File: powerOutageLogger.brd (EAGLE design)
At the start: 99.1 x 74.9 mm, 32 parts, among them J1 2.1MMJACKTHM, U1 ATmega328P, U2 78L05, Y1 16MHz

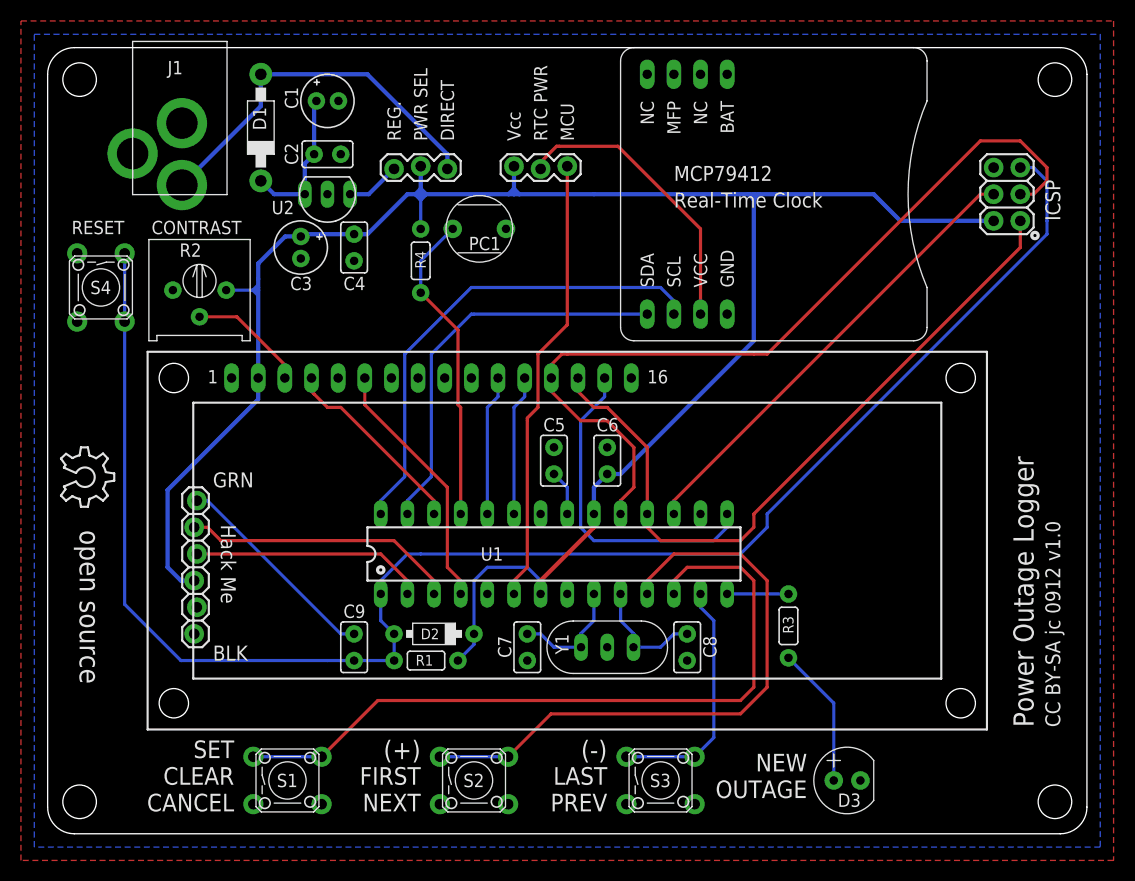
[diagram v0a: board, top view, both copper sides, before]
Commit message: v1.1
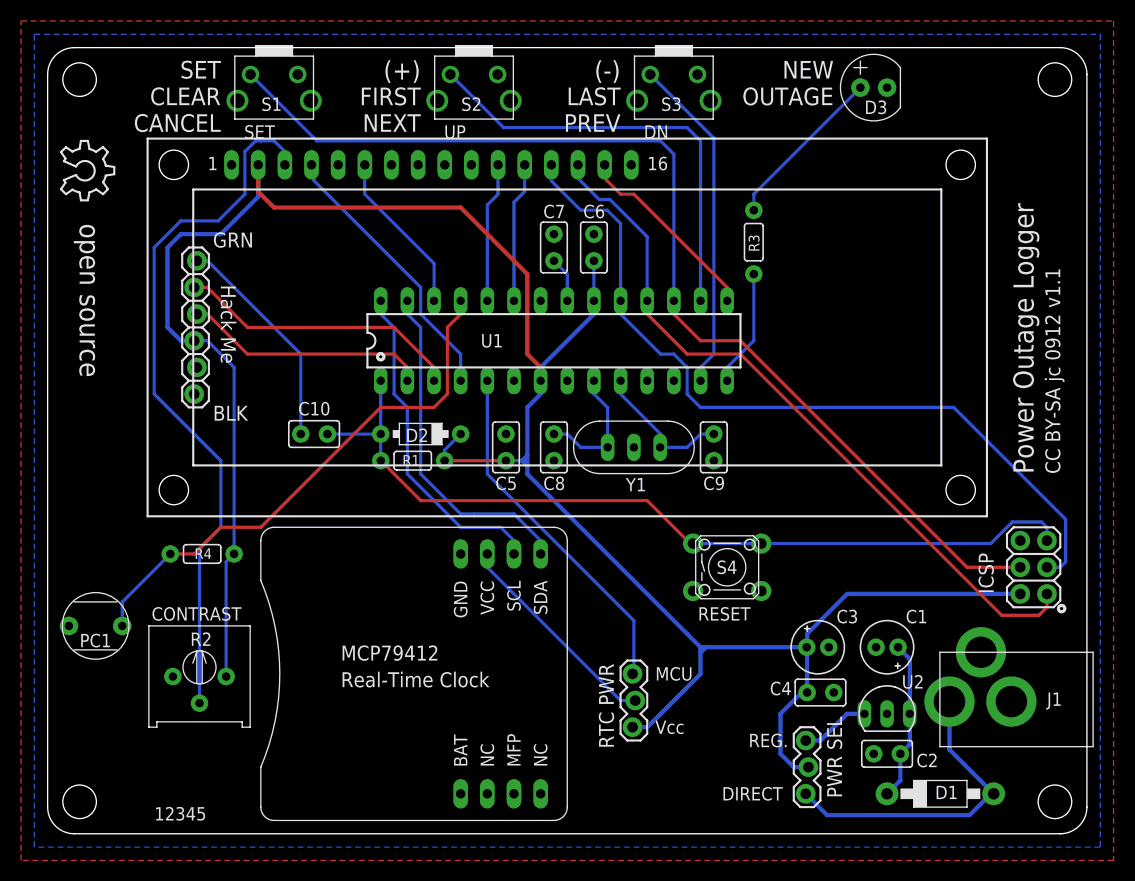
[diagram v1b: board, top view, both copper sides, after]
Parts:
- added C10: 100nF, _jc:C025-025X050
- added U$2: (no value), ohw-logo:OSHW_8X200_NOTEXT
- C7: value 27pF -> 100nF
- C9: value 100nF -> 27pF
- S1, S2: device _jc:B3F-10XXOCT -> _jc:B3F-312X
- S3: value DOWN -> DN; device _jc:B3F-10XXOCT -> _jc:B3F-312X
- moved J1 101.1 mm to (95.2, 12.7), turned to 270 degrees
- moved D1 90.7 mm to (85.1, 3.81), turned to 0 degrees
- moved C2 78.2 mm to (80.0, 7.62), turned to 180 degrees
- moved C1 74.5 mm to (80.0, 17.8), turned to 180 degrees
- moved U2 72.8 mm to (80.0, 11.4), turned to 0 degrees
- moved JP1 68.8 mm to (72.4, 3.81), turned to 90 degrees
- moved D3 66.1 mm to (78.7, 71.1)
- moved S1 66.1 mm to (21.6, 71.1)
- moved S3 66.1 mm to (59.7, 71.1)
- moved S2 66.0 mm to (40.6, 71.1)
- moved S4 65.4 mm to (64.8, 25.4), turned to 0 degrees
- moved C3 62.3 mm to (73.4, 17.8), turned to 0 degrees
- moved C4 61.4 mm to (73.7, 13.5), turned to 0 degrees
- moved PCB1 56.4 mm to (35.6, 15.2), turned to 90 degrees
- moved JP2 54.6 mm to (55.9, 10.2), turned to 90 degrees
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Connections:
- removed net PD4: JP2.3, U1.6
- removed net PD5: S2.1, S2.2, U1.11
- removed net PD6: S1.1, S1.2, U1.12
- net /RESET: now also C10.1; no longer C9.1
- net GND: now also C9.2, S1.1, S2.1, S3.1; no longer S1.3, S1.4, S2.3, S2.4, S3.3, S3.4
- net MOSI: now also S1.2
- net N$9: now also C7.1; no longer C5.1
- net PC3: now also PCB2.6; no longer PCB2.4
- net PD2: now also PCB2.4; no longer PCB2.6
- net PD3: now also JP2.3
- net PD7: no longer S3.1
- net RST: now also C10.2; no longer C9.2
- net SS: now also S2.2
- net VCC: now also C5.1
- net XTAL1: now also C9.1; no longer C8.1
- net XTAL2: now also C8.1; no longer C7.1
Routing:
- net /RESET: track 155.6 -> 81.8 mm
- net PD6: track 70.5 -> 0.00 mm
- net PD5: track 58.9 -> 0.00 mm
- net MOSI: track 43.8 -> 101.8 mm
- net N$3: track 11.3 -> 67.8 mm
- net PD4: track 42.9 -> 0.00 mm
- net SS: track 0.00 -> 41.7 mm
- net PD3: track 0.00 -> 33.9 mm
- net VCC: track 192.7 -> 219.8 mm
- net PC2: track 30.0 -> 50.9 mm
- net SCL: track 46.3 -> 31.6 mm
- net PB1: track 31.5 -> 18.5 mm
- net PD7: track 23.3 -> 32.2 mm
- net N$5: track 27.9 -> 20.6 mm
- net SDA: track 38.3 -> 32.4 mm
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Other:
- board text added: "12345"
- board text added: "CC BY-SA jc 0912 v1.1"
- board text added: "http://github.com/JChristensen"
- board text removed: "CC BY-SA jc 0912 v1.0"
